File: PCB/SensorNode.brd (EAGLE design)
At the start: 58.1 x 69.8 mm, 70 parts, among them J4 USB_MINI-B_SMT, Q1 CMA-4544PF-W, Q2 600mA/40V, Q3 600mA/40V, U1 MAX4466EXK+T, U2 ESP-WROOM-32, U3 Si7021-A20, U4 MCP73831, U5 TSL2561, U6 CP2104, U8 3.3V

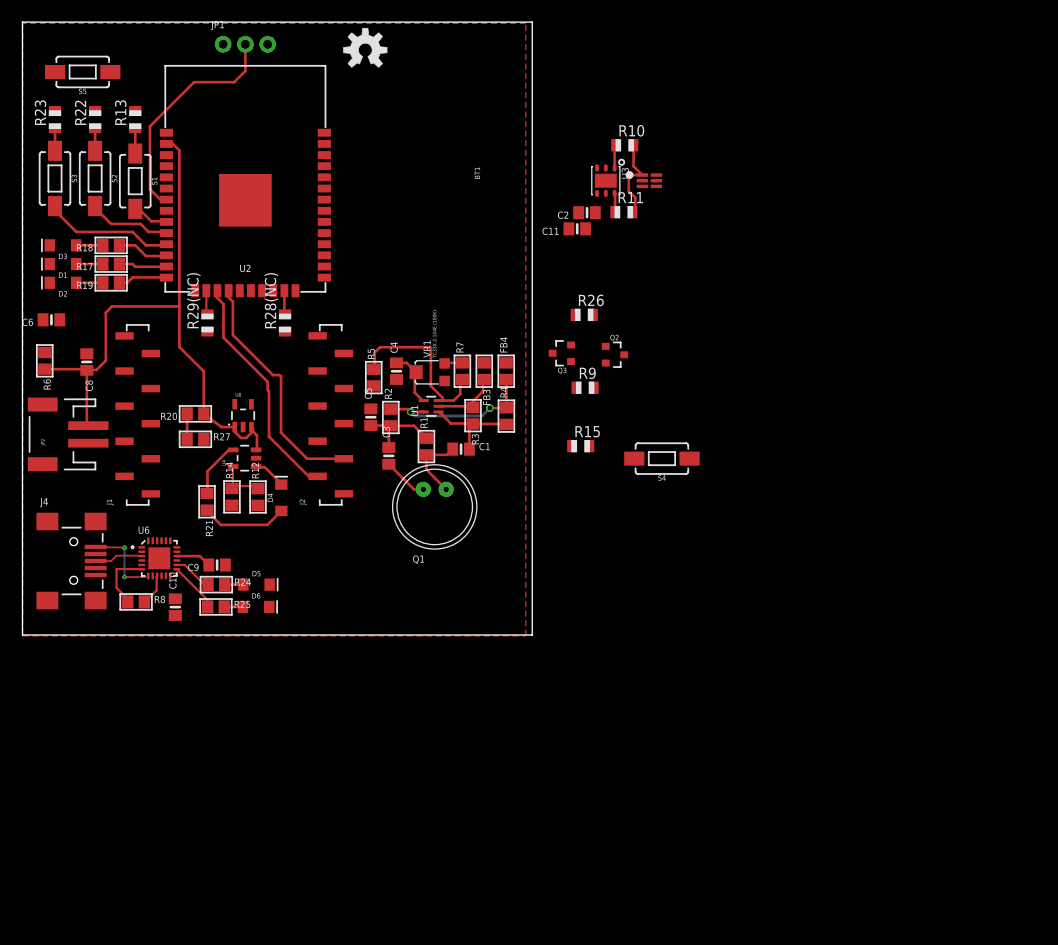
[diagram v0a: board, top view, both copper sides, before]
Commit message: Commit Before AutoRouting
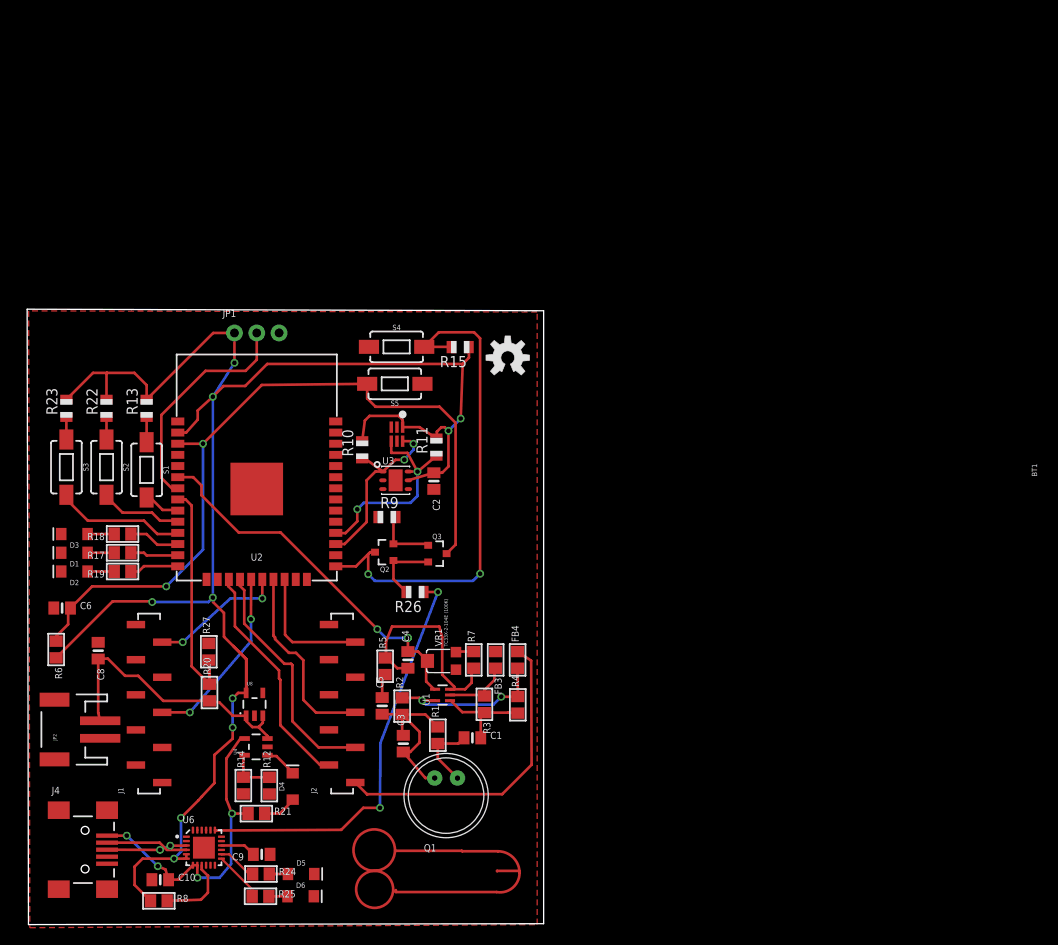
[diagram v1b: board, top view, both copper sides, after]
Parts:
- removed C11: 0.1uF, microbuilder:0805-NO
- removed R28(NC), R29(NC): 0k, adafruit:R0805
- moved BT1 71.9 mm to (62.7, 68.6)
- moved S5 50.3 mm to (41.2, 61.6)
- moved R10 45.8 mm to (37.4, 54.1), turned to 90 degrees
- moved U3 41.7 mm to (41.2, 50.6), turned to 0 degrees
- moved U5 40.8 mm to (41.4, 55.9), turned to 270 degrees
- moved LOGO1 38.6 mm to (54.0, 64.6)
- moved R26 37.0 mm to (43.5, 37.9), turned to 180 degrees
- moved R21 36.0 mm to (25.4, 12.7), turned to 0 degrees
- moved C2 35.2 mm to (45.6, 50.6), turned to 270 degrees
- moved Q2 34.5 mm to (40.0, 42.5), turned to 90 degrees
- moved R11 34.2 mm to (45.9, 54.4), turned to 90 degrees
- moved R8 34.2 mm to (14.3, 2.73)
- moved JP2 33.7 mm to (3.89, 22.3)
- moved C9 33.4 mm to (26.0, 8.03)
- moved D5 33.4 mm to (30.5, 5.79)
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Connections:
- removed net CTS: R28(NC).1, U6.18
- removed net IO13: R29(NC).2, U2.16
- removed net IO15: R28(NC).2, U2.23
- removed net N$16: U2.20
- removed net N$35: R13.1, R22.1, R23.1, S1.1, S2.1, S3.1
- new net N$24: R13.1, S1.1
- new net N$28: R22.1, S2.1
- new net N$29: R23.1, S3.1
- new net N$32: C3.2, R1.2, R2.1
- net AGND: no longer C3.2, R1.2, R2.1
- net CTS1: now also U2.20
- net GND: no longer C11.2
- net IO7: now also U2.21
- net IO8: no longer U2.21
- net RTS: no longer R29(NC).1, U6.20
- net TXD0: now also U6.20
- net VCC: now also FB4.2, J2.1, JP1.1, R10.2, R11.2, R6.2, U2.2, U5.VDD
- net VCC_3.7V: no longer C11.1, FB4.2, J2.1, JP1.1, R10.2, R11.2, R6.2, U2.2, U5.VDD
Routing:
- net VCC: track 7.17 -> 233.4 mm, vias 0 -> 10
- net EN: track 0.00 -> 87.0 mm, vias 0 -> 2
- net IO0: track 0.00 -> 58.1 mm, vias 0 -> 2
- net RTS: track 0.00 -> 47.3 mm, vias 0 -> 2
- net VCC_3.7V: track 78.7 -> 32.3 mm
- net IO34: track 6.45 -> 42.5 mm, vias 0 -> 2
- net N$16: track 0.00 -> 30.3 mm
- net IO32: track 2.90 -> 28.4 mm
- net IO7: track 0.00 -> 22.1 mm
- net SCL: track 2.16 -> 24.1 mm, vias 0 -> 2
- net VBUS: track 15.6 -> 36.6 mm, vias 2 -> 4
- net RTS1: track 0.00 -> 21.0 mm, vias 0 -> 2
- net SDA: track 2.65 -> 20.9 mm, vias 0 -> 2
- net CTS1: track 0.00 -> 15.5 mm, vias 0 -> 2
- net IO8: track 0.00 -> 14.7 mm
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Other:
- board size 58.1 x 69.8 mm -> 58.9 x 70.1 mm
